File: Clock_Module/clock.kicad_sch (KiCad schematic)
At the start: 28 parts, among them SW1 Switch, U1 74LS08, U2 74LS32, U3 74LS04, U4 LM555xN, U5 LM555xN, U6 LM555xN

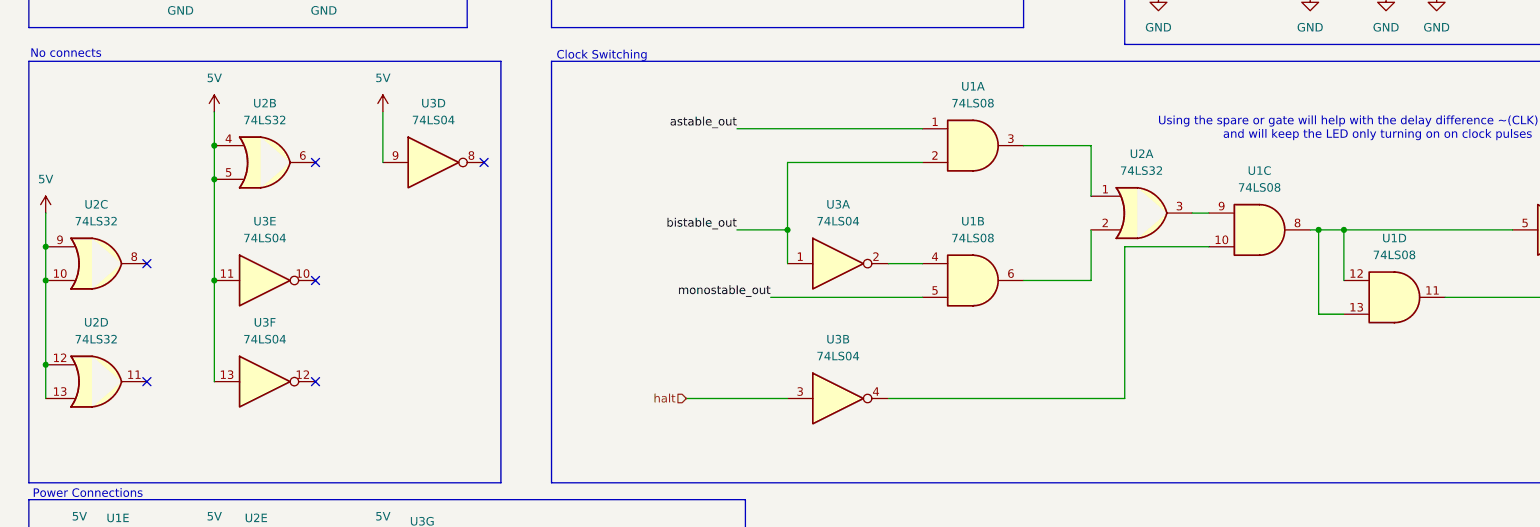
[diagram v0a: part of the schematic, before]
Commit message: sim going through major revisions
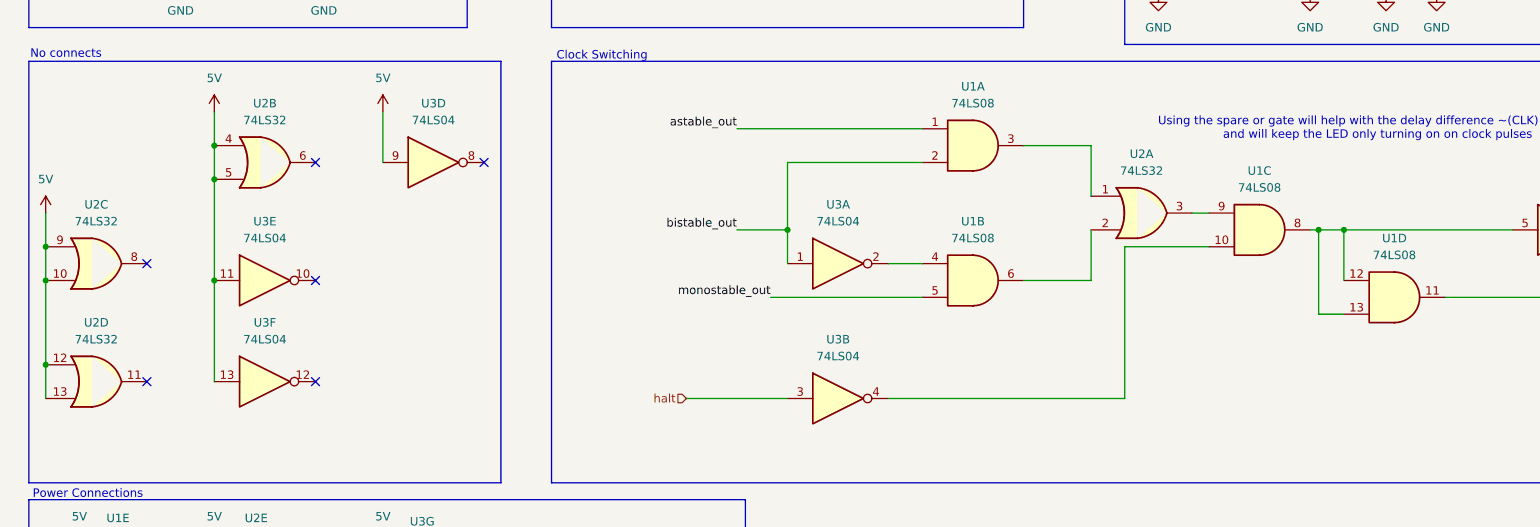
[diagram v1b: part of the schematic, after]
